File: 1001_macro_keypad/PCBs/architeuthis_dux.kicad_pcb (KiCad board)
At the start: 2 copper layers, 32 parts, among them J1 ePaperModule, J2 RotaryModule_01, J3 RotaryModule_02, SW01 MX_SW, SW10 MX_SW, SW11 MX_SW, SW12 MX_SW, SW13 MX_SW, SW14 MX_SW, SW2 MX_SW, SW3 MX_SW, SW4 MX_SW, SW5 MX_SW, SW6 MX_SW, SW7 MX_SW, SW8 MX_SW, SW9 MX_SW, U1 Pico

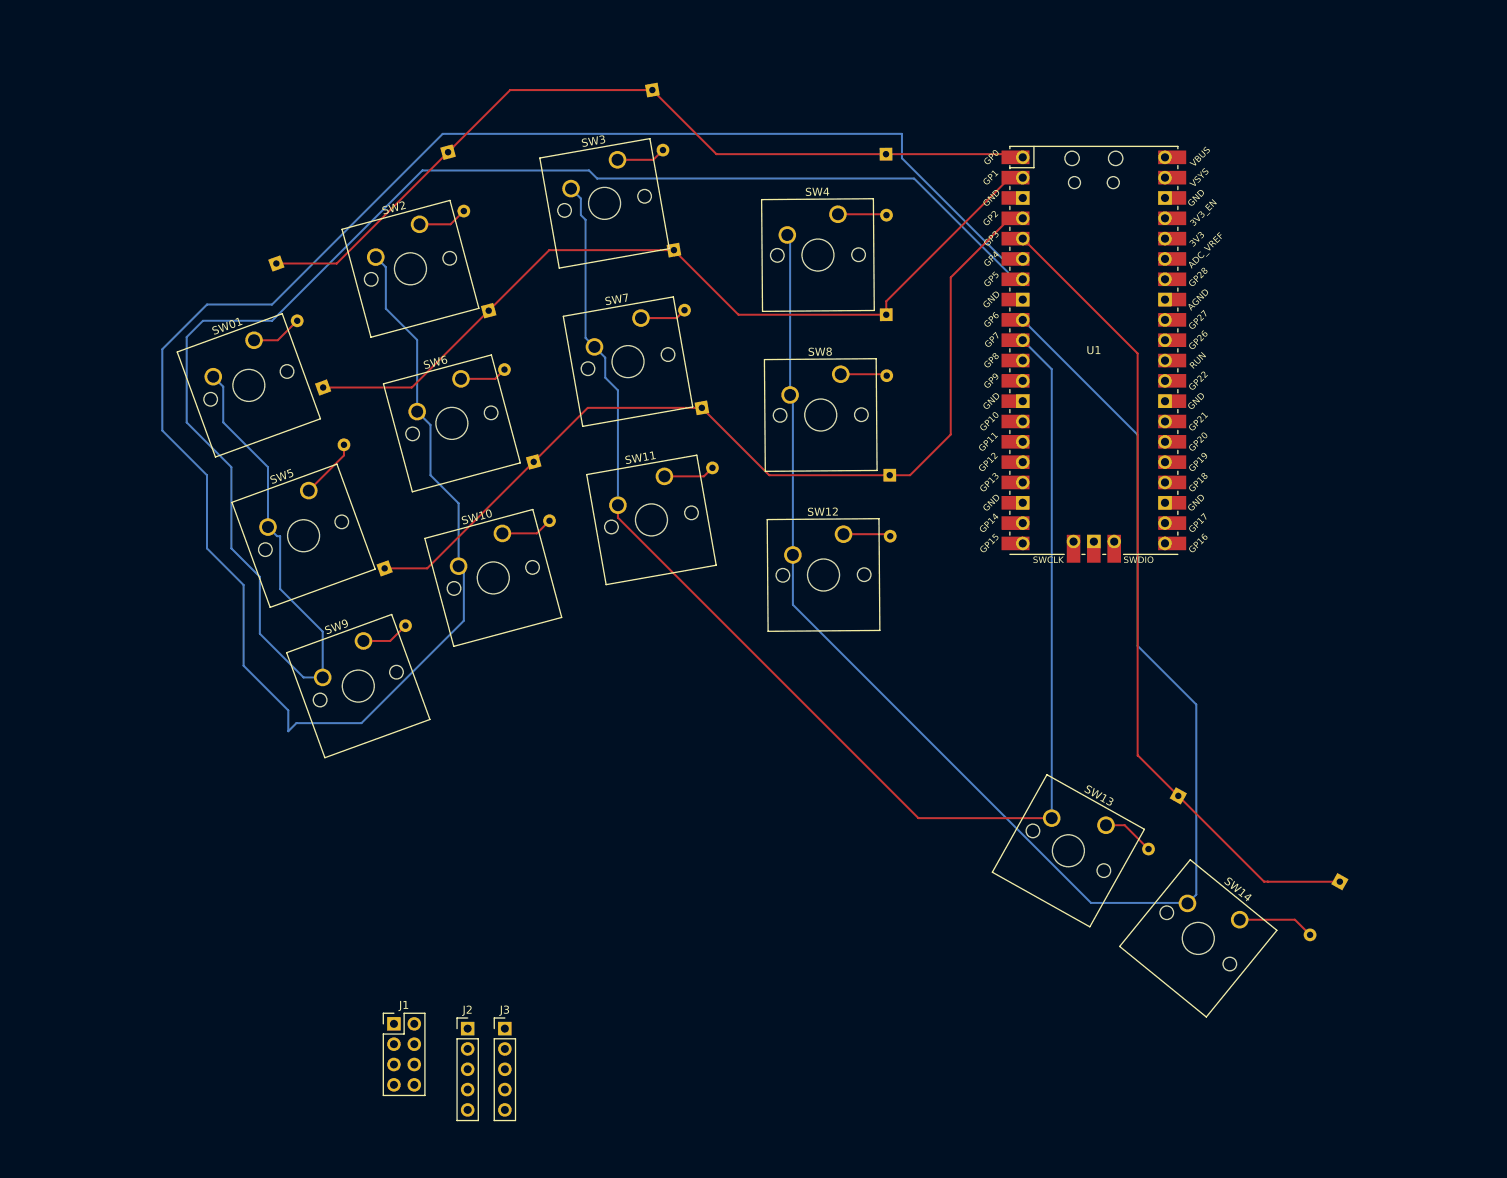
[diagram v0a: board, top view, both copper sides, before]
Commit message: 재배선
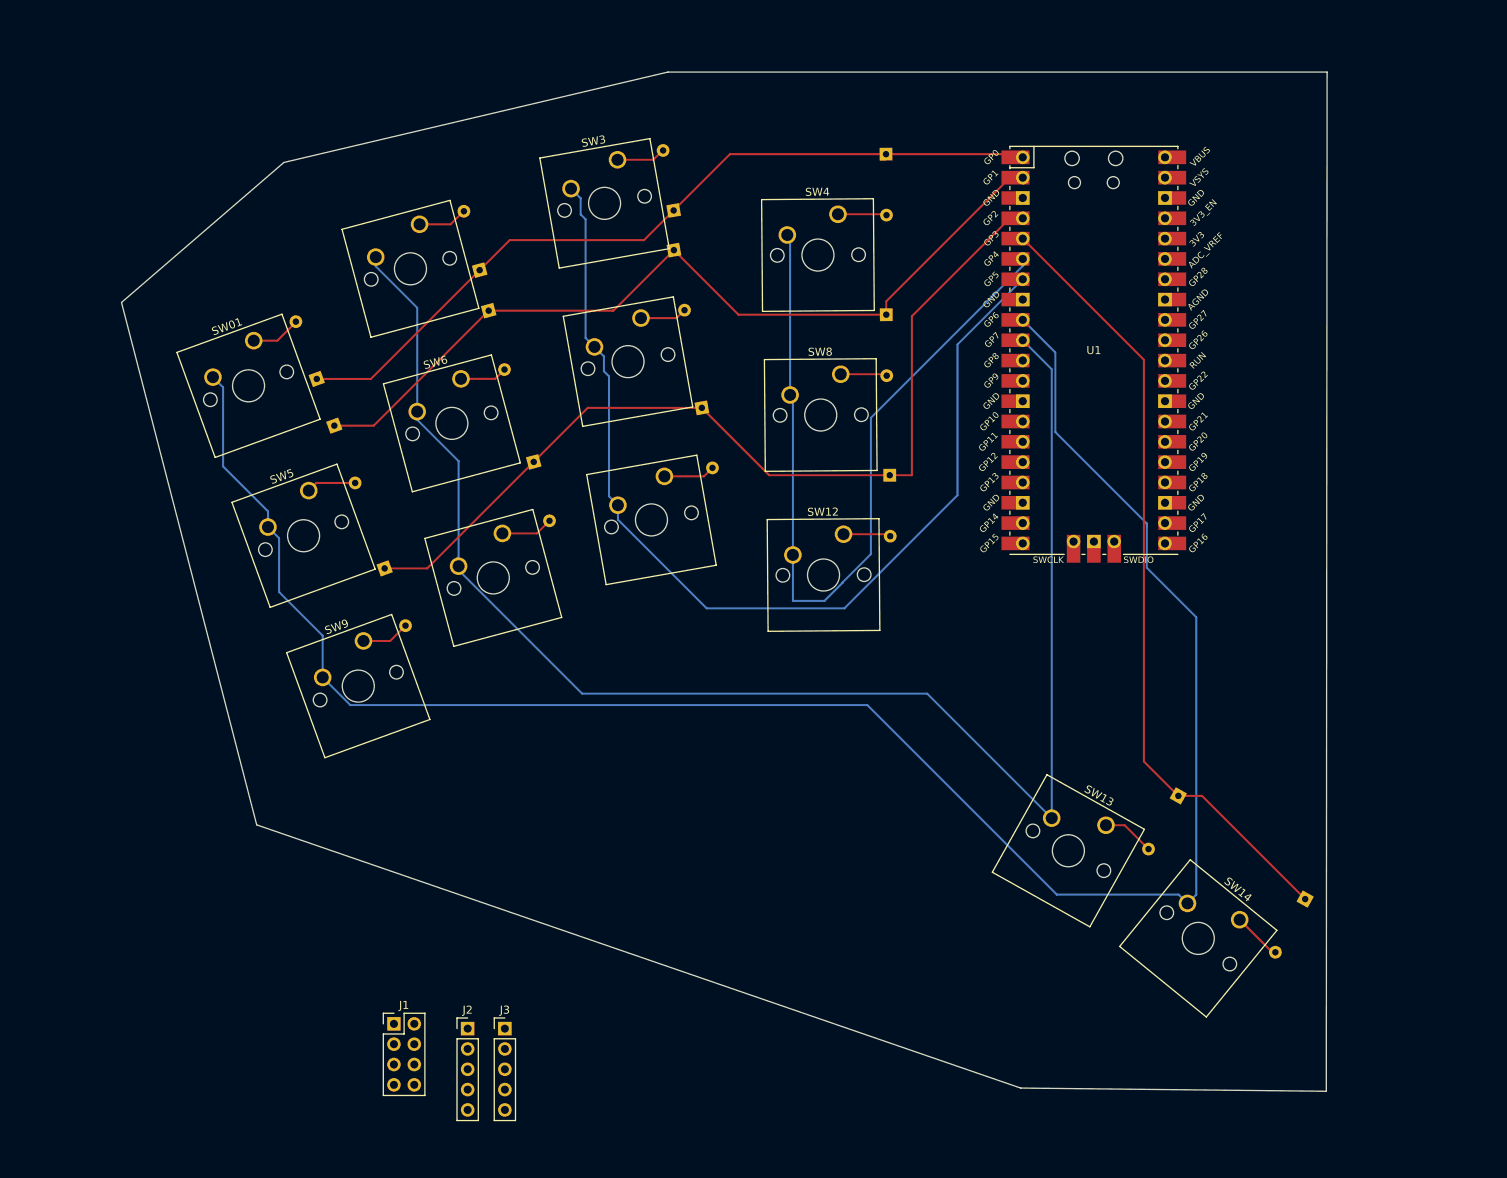
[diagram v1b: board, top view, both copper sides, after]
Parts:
- moved D1 15.3 mm to (146.3, 70.3), turned to 110 degrees
- moved D3 15.3 mm to (190.9, 49.2), turned to 100 degrees
- moved D2 15.3 mm to (166.7, 56.7), turned to 105 degrees
- moved D5 4.97 mm to (148.5, 76.1)
- moved D14 4.85 mm to (269.9, 135.3)
- moved SW01 0.07 mm to (138.4, 65.5)
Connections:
- SW01 pad 2: COL0 -> COL2
- SW10 pad 2: COL1 -> COL3
- SW11 pad 2: COL2 -> COL1
- SW12 pad 2: COL3 -> COL0
- SW13 pad 2: COL2 -> COL3
- SW14 pad 2: COL3 -> COL2
- SW2 pad 2: COL1 -> COL3
- SW3 pad 2: COL2 -> COL1
- SW4 pad 2: COL3 -> COL0
- SW5 pad 2: COL0 -> COL2
- SW6 pad 2: COL1 -> COL3
- SW7 pad 2: COL2 -> COL1
- SW8 pad 2: COL3 -> COL0
- SW9 pad 2: COL0 -> COL2
- U1 pad 10: COL2 -> COL3
- U1 pad 6: COL1 -> COL0
- U1 pad 7: COL0 -> COL1
- U1 pad 9: COL3 -> COL2
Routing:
- net COL1: track 258.9 -> 128.1 mm
- net COL0: track 213.2 -> 103.0 mm
- net COL2: track 174.6 -> 245.9 mm
- net ROW0: track 107.5 -> 100.6 mm
- net ROW3: track 102.4 -> 98.9 mm
- net Net-(D14-A): track 9.58 -> 6.15 mm
- net Net-(D5-A): track 7.55 -> 6.20 mm
- net COL3: track 193.7 -> 192.8 mm
- net ROW1: track 106.0 -> 106.6 mm
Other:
- board outline added: 150.7 x 127.4 mm

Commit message: ePaper
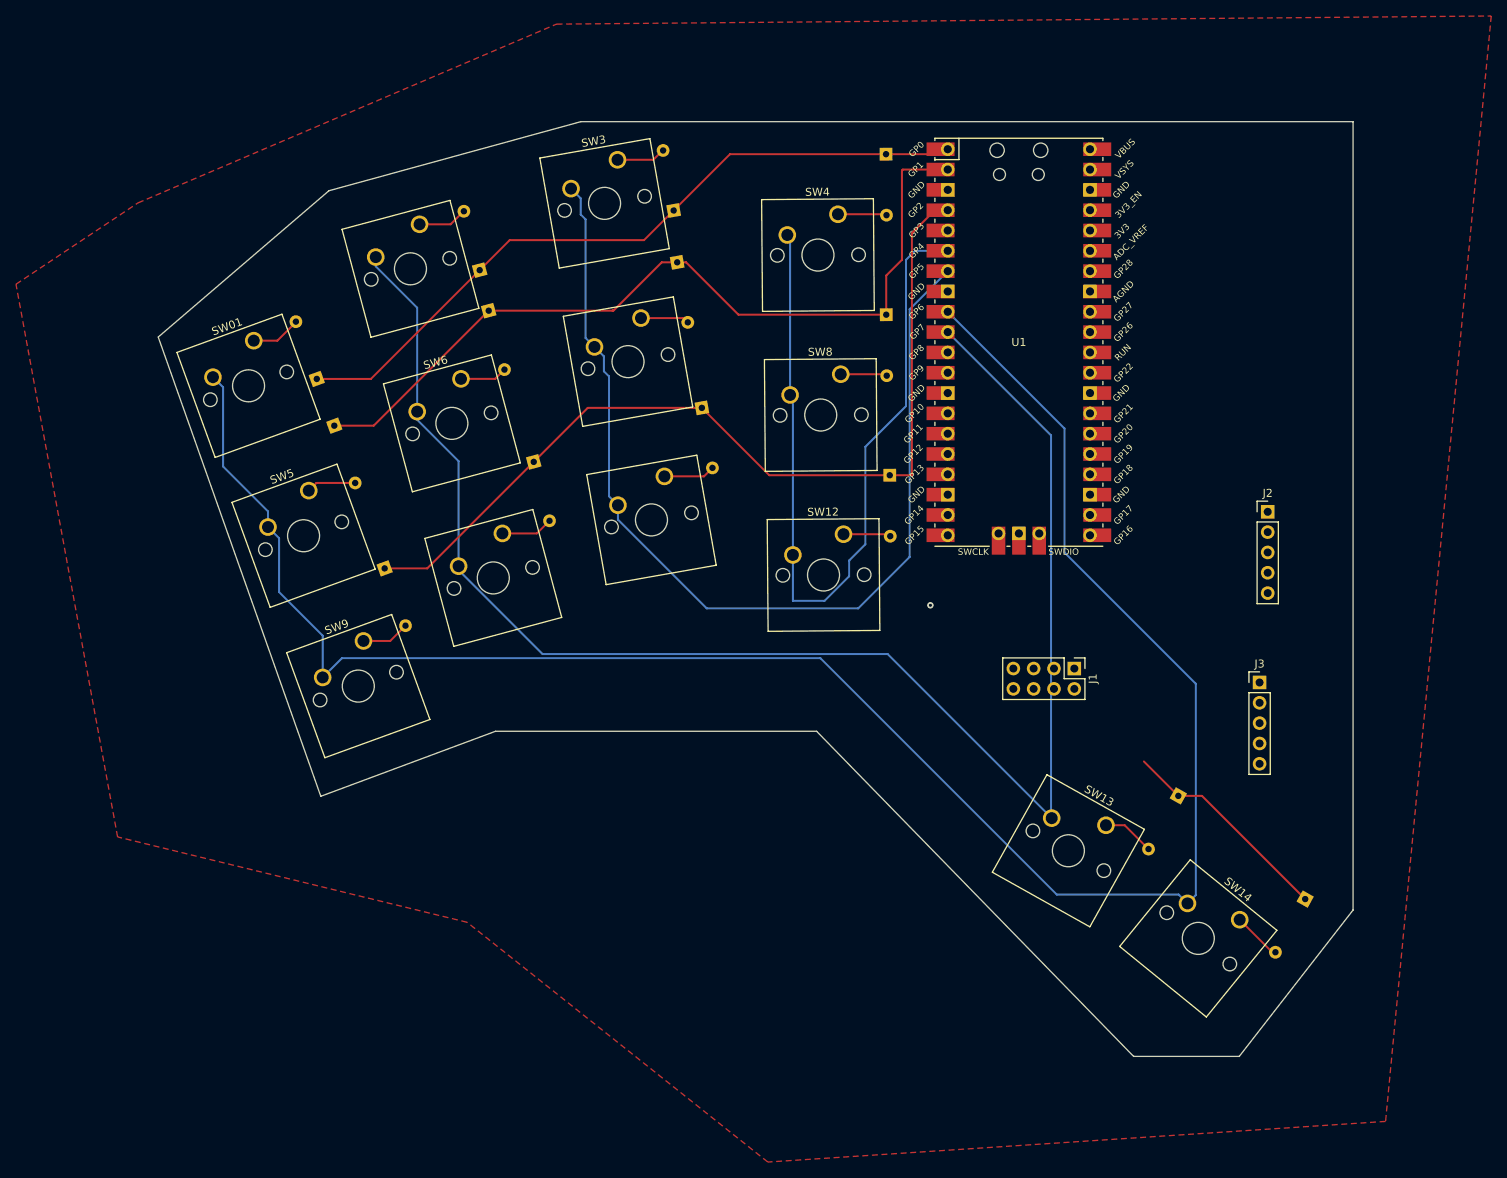
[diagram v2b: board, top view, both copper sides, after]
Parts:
- moved J2 119.1 mm to (265.2, 86.9)
- moved J3 103.8 mm to (264.2, 108.2)
- moved J1 95.9 mm to (241.0, 106.5), turned to -90 degrees
- moved U1 9.43 mm to (234.1, 65.7)
- moved D7 1.58 mm to (191.4, 55.7)
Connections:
- J1 pad 7: unconnected-(J1-Pin_7-Pad7) -> GND
- J1 pad 8: unconnected-(J1-Pin_8-Pad8) -> +5V
- J2 pad 1: unconnected-(J2-Pin_1-Pad1) -> +5V
- J2 pad 5: unconnected-(J2-Pin_5-Pad5) -> GND
- J3 pad 1: unconnected-(J3-Pin_1-Pad1) -> +5V
- J3 pad 5: unconnected-(J3-Pin_5-Pad5) -> GND
- U1 pad 40: unconnected-(U1-VBUS-Pad40) -> +5V
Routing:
- net ROW3: track 98.9 -> 27.3 mm
- net ROW0: track 100.6 -> 90.8 mm
- net COL2: track 245.9 -> 252.2 mm
- net COL3: track 192.8 -> 196.5 mm
- net ROW2: track 116.5 -> 113.6 mm
- net COL1: track 128.1 -> 125.2 mm
- net ROW1: track 106.6 -> 104.8 mm
- net (no net): vias 0 -> 1
- added copper zone on F.Cu, net GND
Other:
- board size 150.7 x 127.4 mm -> 149.4 x 116.8 mm
